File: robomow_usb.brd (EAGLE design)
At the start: 17.8 x 42 mm, 25 parts, among them IC1 FT231XS-R, J1 RJ11-2L-B, U1 SN65HVD1176

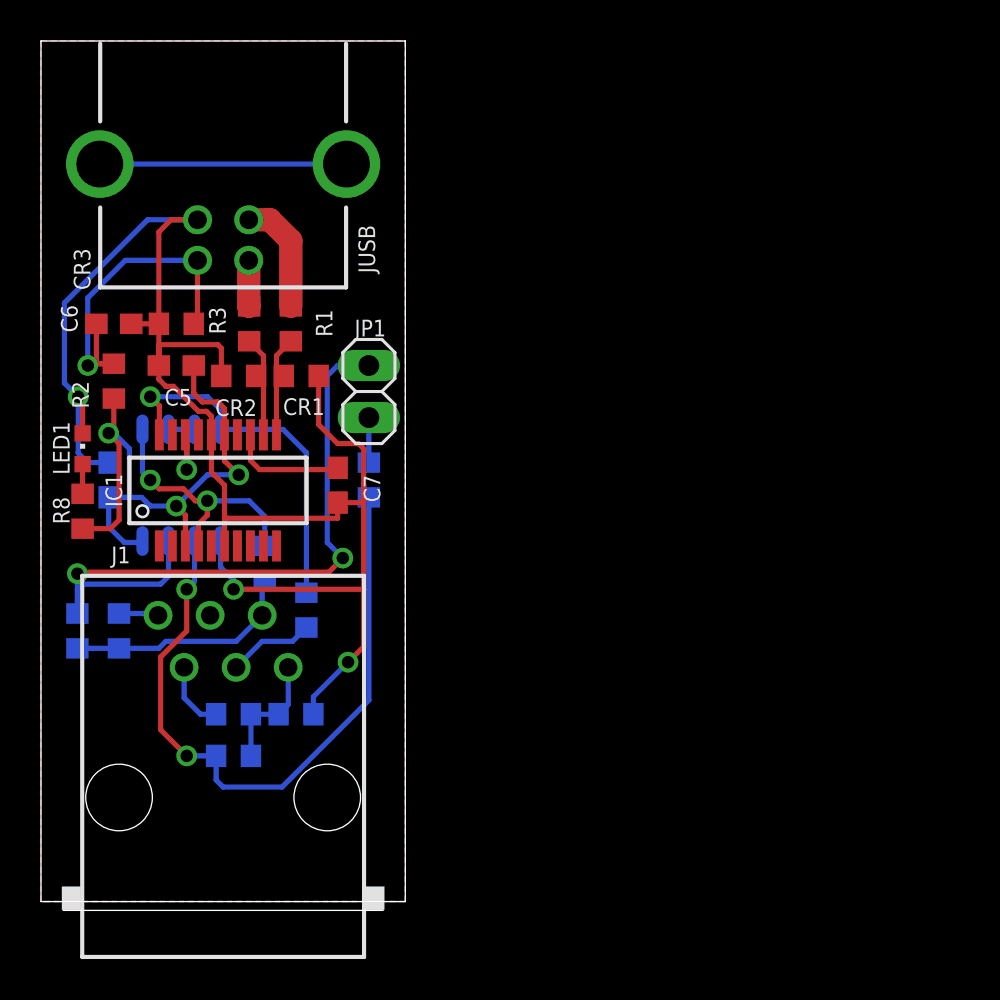
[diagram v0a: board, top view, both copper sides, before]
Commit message: Polish routing
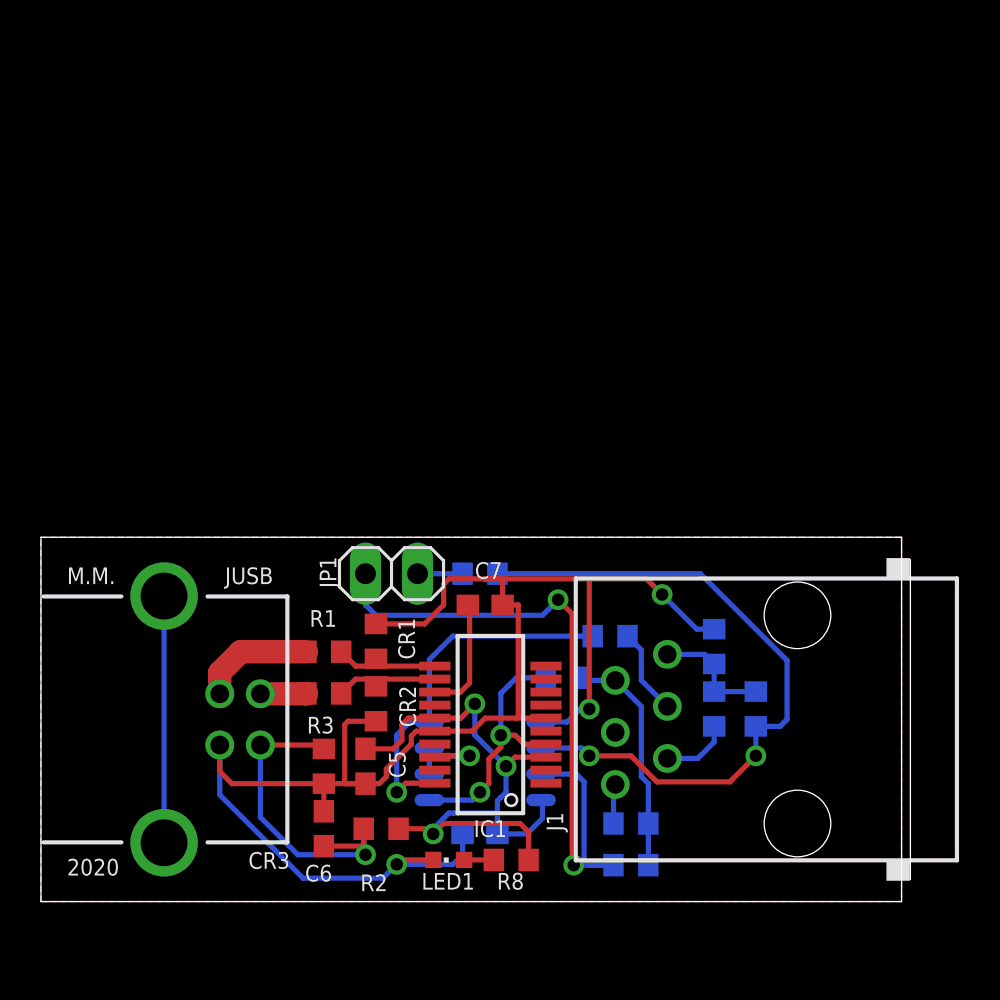
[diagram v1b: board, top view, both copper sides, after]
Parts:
- moved R12 29.3 mm to (28.8, 1.78), turned to 0 degrees
- moved J1 28.3 mm to (36.9, 8.89), turned to 90 degrees
- moved R8 27.0 mm to (22.9, 2.03), turned to 180 degrees
- moved LED1 26.9 mm to (19.9, 2.03), turned to 90 degrees
- moved R4 26.7 mm to (28.8, 3.81), turned to 0 degrees
- moved C6 26.7 mm to (13.8, 3.56), turned to 90 degrees
- moved R11 25.6 mm to (34.9, 9.40), turned to 270 degrees
- moved R2 25.4 mm to (16.6, 3.56), turned to 0 degrees
- moved C1 25.0 mm to (21.4, 3.30), turned to 0 degrees
- moved JUSB 24.4 mm to (8.73, 8.89), turned to 0 degrees
- moved R10 23.5 mm to (32.9, 9.40), turned to 270 degrees
- moved CR3 22.8 mm to (13.8, 6.60), turned to 90 degrees
- moved C5 21.6 mm to (15.8, 6.60), turned to 270 degrees
- moved R9 20.7 mm to (32.9, 12.4), turned to 90 degrees
- moved U1 20.0 mm to (21.7, 6.86), turned to 180 degrees
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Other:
- board size 17.8 x 42 mm -> 42 x 17.8 mm
- board text added: "2020"
- board text added: "M.M."
